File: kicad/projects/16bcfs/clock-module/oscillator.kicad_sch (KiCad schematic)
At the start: 10 parts, among them SW1 SW_SPST, SW2 SW_SPST, SW3 SW_SPST, SW4 SW_SPST, U7 74HC193, X1 XO32

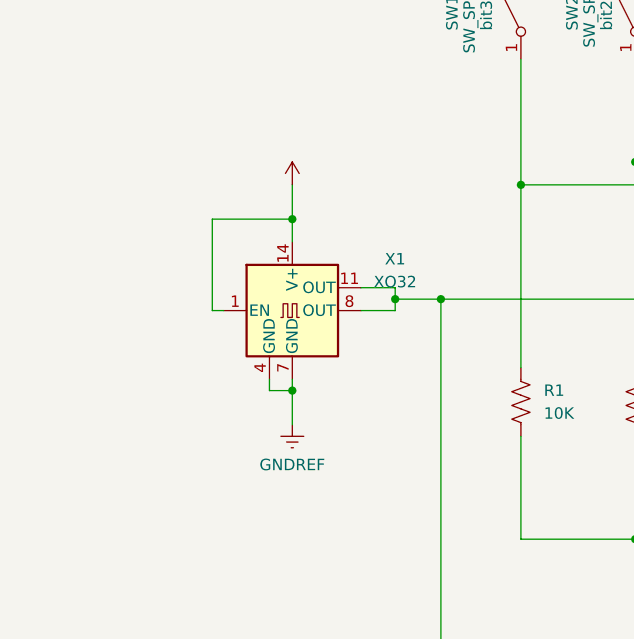
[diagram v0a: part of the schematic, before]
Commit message: Some KiCad Cleanup
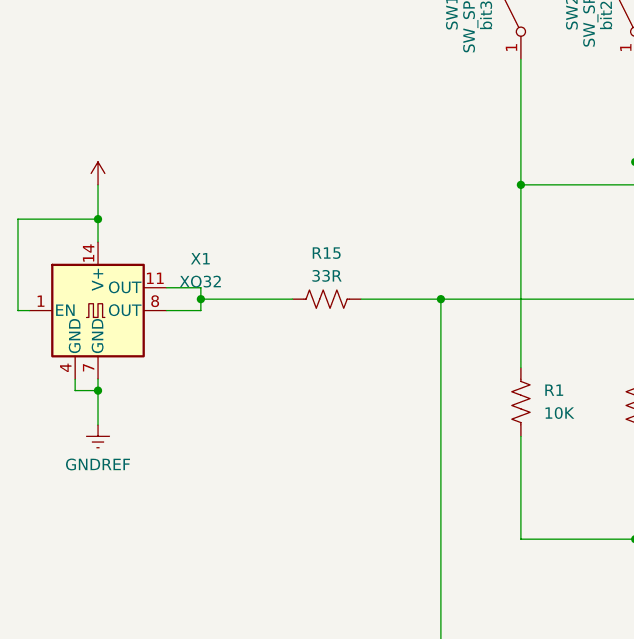
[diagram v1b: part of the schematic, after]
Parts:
- added R15: 33R, symbol Device:R_US
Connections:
- net HS_CLK: now also R15.2; no longer X1.11 (OUT), X1.8 (OUT)
- new net: R15.1, X1.11 (OUT), X1.8 (OUT)
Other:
- moved on the sheet: X1
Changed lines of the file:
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@@
   (junction (at 144.78 53.34) (diameter 0) (color 0 0 0 0)
   )
-  (junction (at 81.28 106.68) (diameter 0) (color 0 0 0 0)
+  (junction (at 59.69 106.68) (diameter 0) (color 0 0 0 0)
   )
   (junction (at 97.79 96.52) (diameter 0) (color 0 0 0 0)
@@
   (junction (at 132.08 78.74) (diameter 0) (color 0 0 0 0)
   )
-  (junction (at 81.28 87.63) (diameter 0) (color 0 0 0 0)
+  (junction (at 59.69 87.63) (diameter 0) (color 0 0 0 0)
   )
   (junction (at 144.78 123.19) (diameter 0) (color 0 0 0 0)
   )
-  (junction (at 92.71 96.52) (diameter 0) (color 0 0 0 0)
+  (junction (at 71.12 96.52) (diameter 0) (color 0 0 0 0)
   )
   (junction (at 180.34 123.19) (diameter 0) (color 0 0 0 0)
@@
   (no_connect (at 193.04 83.82))
   (no_connect (at 193.04 88.9))
-  (wire (pts (xy 72.39 97.79) (xy 72.39 87.63))
-    (stroke (width 0) (type default))
-  )
-  (wire (pts (xy 92.71 96.52) (xy 97.79 96.52))
+  (wire (pts (xy 50.8 97.79) (xy 50.8 87.63))
+    (stroke (width 0) (type default))
+  )
+  (wire (pts (xy 71.12 96.52) (xy 81.28 96.52))
     (stroke (width 0) (type default))
   )
@@
     (stroke (width 0) (type default))
   )
-  (wire (pts (xy 73.66 97.79) (xy 72.39 97.79))
+  (wire (pts (xy 52.07 97.79) (xy 50.8 97.79))
     (stroke (width 0) (type default))
   )
@@
     (stroke (width 0) (type default))
   )
-  (wire (pts (xy 72.39 87.63) (xy 81.28 87.63))
+  (wire (pts (xy 50.8 87.63) (xy 59.69 87.63))
     (stroke (width 0) (type default))
   )
@@
     (stroke (width 0) (type default))
   )
-  (wire (pts (xy 88.9 95.25) (xy 92.71 95.25))
+  (wire (pts (xy 67.31 95.25) (xy 71.12 95.25))
     (stroke (width 0) (type default))
   )
@@
     (stroke (width 0) (type default))
   )
-  (wire (pts (xy 78.74 105.41) (xy 78.74 106.68))
+  (wire (pts (xy 57.15 105.41) (xy 57.15 106.68))
     (stroke (width 0) (type default))
   )
@@
     (stroke (width 0) (type default))
   )
-  (wire (pts (xy 81.28 83.82) (xy 81.28 87.63))
+  (wire (pts (xy 59.69 83.82) (xy 59.69 87.63))
     (stroke (width 0) (type default))
   )
@@
     (stroke (width 0) (type default))
   )
-  (wire (pts (xy 81.28 110.49) (xy 81.28 106.68))
+  (wire (pts (xy 59.69 110.49) (xy 59.69 106.68))
     (stroke (width 0) (type default))
   )
@@
     (stroke (width 0) (type default))
   )
-  (wire (pts (xy 78.74 106.68) (xy 81.28 106.68))
+  (wire (pts (xy 57.15 106.68) (xy 59.69 106.68))
     (stroke (width 0) (type default))
   )
@@
     (stroke (width 0) (type default))
   )
-  (wire (pts (xy 92.71 95.25) (xy 92.71 96.52))
+  (wire (pts (xy 71.12 95.25) (xy 71.12 96.52))
     (stroke (width 0) (type default))
   )
@@
     (stroke (width 0) (type default))
   )
-  (wire (pts (xy 92.71 97.79) (xy 88.9 97.79))
-    (stroke (width 0) (type default))
-  )
-  (wire (pts (xy 92.71 97.79) (xy 92.71 96.52))
+  (wire (pts (xy 71.12 97.79) (xy 67.31 97.79))
+    (stroke (width 0) (type default))
+  )
+  (wire (pts (xy 71.12 97.79) (xy 71.12 96.52))
     (stroke (width 0) (type default))
   )
@@
     (stroke (width 0) (type default))
   )
+  (wire (pts (xy 88.9 96.52) (xy 97.79 96.52))
+    (stroke (width 0) (type default))
+  )
   (wire (pts (xy 167.64 93.98) (xy 163.83 93.98))
     (stroke (width 0) (type default))
@@
     (stroke (width 0) (type default))
   )
-  (wire (pts (xy 81.28 87.63) (xy 81.28 90.17))
+  (wire (pts (xy 59.69 87.63) (xy 59.69 90.17))
     (stroke (width 0) (type default))
   )
@@
     (stroke (width 0) (type default))
   )
-  (wire (pts (xy 81.28 106.68) (xy 81.28 105.41))
+  (wire (pts (xy 59.69 106.68) (xy 59.69 105.41))
     (stroke (width 0) (type default))
   )
@@
     )
   )
-  (symbol (lib_id "eryjus:XO32-Dual") (at 81.28 97.79 0) (unit 1)
+  (symbol (lib_id "eryjus:XO32-Dual") (at 59.69 97.79 0) (unit 1)
     (in_bom yes) (on_board yes) (dnp no)
-    (property "Reference" "X1" (at 92.71 92.075 0)
-      (effects (font (size 1.27 1.27)))
-    )
-    (property "Value" "XO32" (at 92.71 94.615 0)
-      (effects (font (size 1.27 1.27)))
-    )
-    (property "Footprint" "eryjus:Oscillator_DIP-8-14" (at 99.06 106.68 0)
-      (effects (font (size 1.27 1.27)) hide)
-    )
-    (property "Datasheet" "http://cdn-reichelt.de/documents/datenblatt/B400/XO32.pdf" (at 78.74 97.79 0)
+    (property "Reference" "X1" (at 71.12 92.075 0)
+      (effects (font (size 1.27 1.27)))
+    )
+    (property "Value" "XO32" (at 71.12 94.615 0)
+      (effects (font (size 1.27 1.27)))
+    )
+    (property "Footprint" "eryjus:Oscillator_DIP-8-14" (at 77.47 106.68 0)
+      (effects (font (size 1.27 1.27)) hide)
+    )
+    (property "Datasheet" "http://cdn-reichelt.de/documents/datenblatt/B400/XO32.pdf" (at 57.15 97.79 0)
       (effects (font (size 1.27 1.27)) hide)
     )
@@
     )
   )
-  (symbol (lib_id "power:GNDREF") (at 81.28 110.49 0) (unit 1)
+  (symbol (lib_id "Device:R_US") (at 85.09 96.52 90) (unit 1)
+    (in_bom yes) (on_board yes) (dnp no)
+    (property "Reference" "R15" (at 85.09 91.44 90)
+      (effects (font (size 1.27 1.27)))
+    )
+    (property "Value" "33R" (at 85.09 93.98 90)
+      (effects (font (size 1.27 1.27)))
+    )
+    (property "Footprint" "" (at 85.344 95.504 90)
+      (effects (font (size 1.27 1.27)) hide)
+    )
+    (property "Datasheet" "~" (at 85.09 96.52 0)
+      (effects (font (size 1.27 1.27)) hide)
+    )
+    (pin "2")
+    (pin "1")
+    (instances
+      (project "clock-module"
+        (path "/d0ae44e5-d74e-4df6-bf3d-e0535c5a7785/17247281-d2e9-42e8-adcf-c7e0678ef791"
+          (reference "R15") (unit 1)
+        )
+      )
+    )
+  )
+  (symbol (lib_id "power:GNDREF") (at 59.69 110.49 0) (unit 1)
     (in_bom yes) (on_board yes) (dnp no) (fields_autoplaced)
-    (property "Reference" "#PWR05" (at 81.28 116.84 0)
-      (effects (font (size 1.27 1.27)) hide)
-    )
-    (property "Value" "GNDREF" (at 81.28 114.935 0)
-      (effects (font (size 1.27 1.27)))
-    )
-    (property "Footprint" "" (at 81.28 110.49 0)
-      (effects (font (size 1.27 1.27)) hide)
-    )
-    (property "Datasheet" "" (at 81.28 110.49 0)
+    (property "Reference" "#PWR05" (at 59.69 116.84 0)
+      (effects (font (size 1.27 1.27)) hide)
+    )
+    (property "Value" "GNDREF" (at 59.69 114.935 0)
+      (effects (font (size 1.27 1.27)))
+    )
+    (property "Footprint" "" (at 59.69 110.49 0)
+      (effects (font (size 1.27 1.27)) hide)
+    )
+    (property "Datasheet" "" (at 59.69 110.49 0)
       (effects (font (size 1.27 1.27)) hide)
     )
@@
     )
   )
-  (symbol (lib_id "power:VCC") (at 81.28 83.82 0) (unit 1)
+  (symbol (lib_id "power:VCC") (at 59.69 83.82 0) (unit 1)
     (in_bom yes) (on_board yes) (dnp no) (fields_autoplaced)
-    (property "Reference" "#PWR04" (at 81.28 87.63 0)
-      (effects (font (size 1.27 1.27)) hide)
-    )
-    (property "Value" "VCC" (at 81.28 79.375 0)
-      (effects (font (size 1.27 1.27)) hide)
-    )
-    (property "Footprint" "" (at 81.28 83.82 0)
-      (effects (font (size 1.27 1.27)) hide)
-    )
-    (property "Datasheet" "" (at 81.28 83.82 0)
-      (effects (font (size 1.27 1.27)) hide)
-    )
+    (property "Reference" "#PWR04" (at 59.69 87.63 0)
+      (effects (font (size 1.27 1.27)) hide)
+    )
+    (property "Value" "VCC" (at 59.69 79.375 0)
+      (effects (font (size 1.27 1.27)) hide)
+    )
+    (property "Footprint" "" (at 59.69 83.82 0)
+      (effects (font (size 1.27 1.27)) hide)
+    )
+    (property "Datasheet" "" (at 59.69 83.82 0)
+      (effects (font (size 1.27 1.27)) hide)
+    )
